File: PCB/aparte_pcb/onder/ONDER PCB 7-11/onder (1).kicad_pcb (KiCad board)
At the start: 2 copper layers, 170 x 170 mm, 77 parts, among them J1 Conn_01x04_Socket, J2 Conn_01x10_Socket, J3 Screw_Terminal_01x01, J4 Screw_Terminal_01x01, J5 Screw_Terminal_01x01, Q1 NPN, Q2 NPN, Q3 NPN

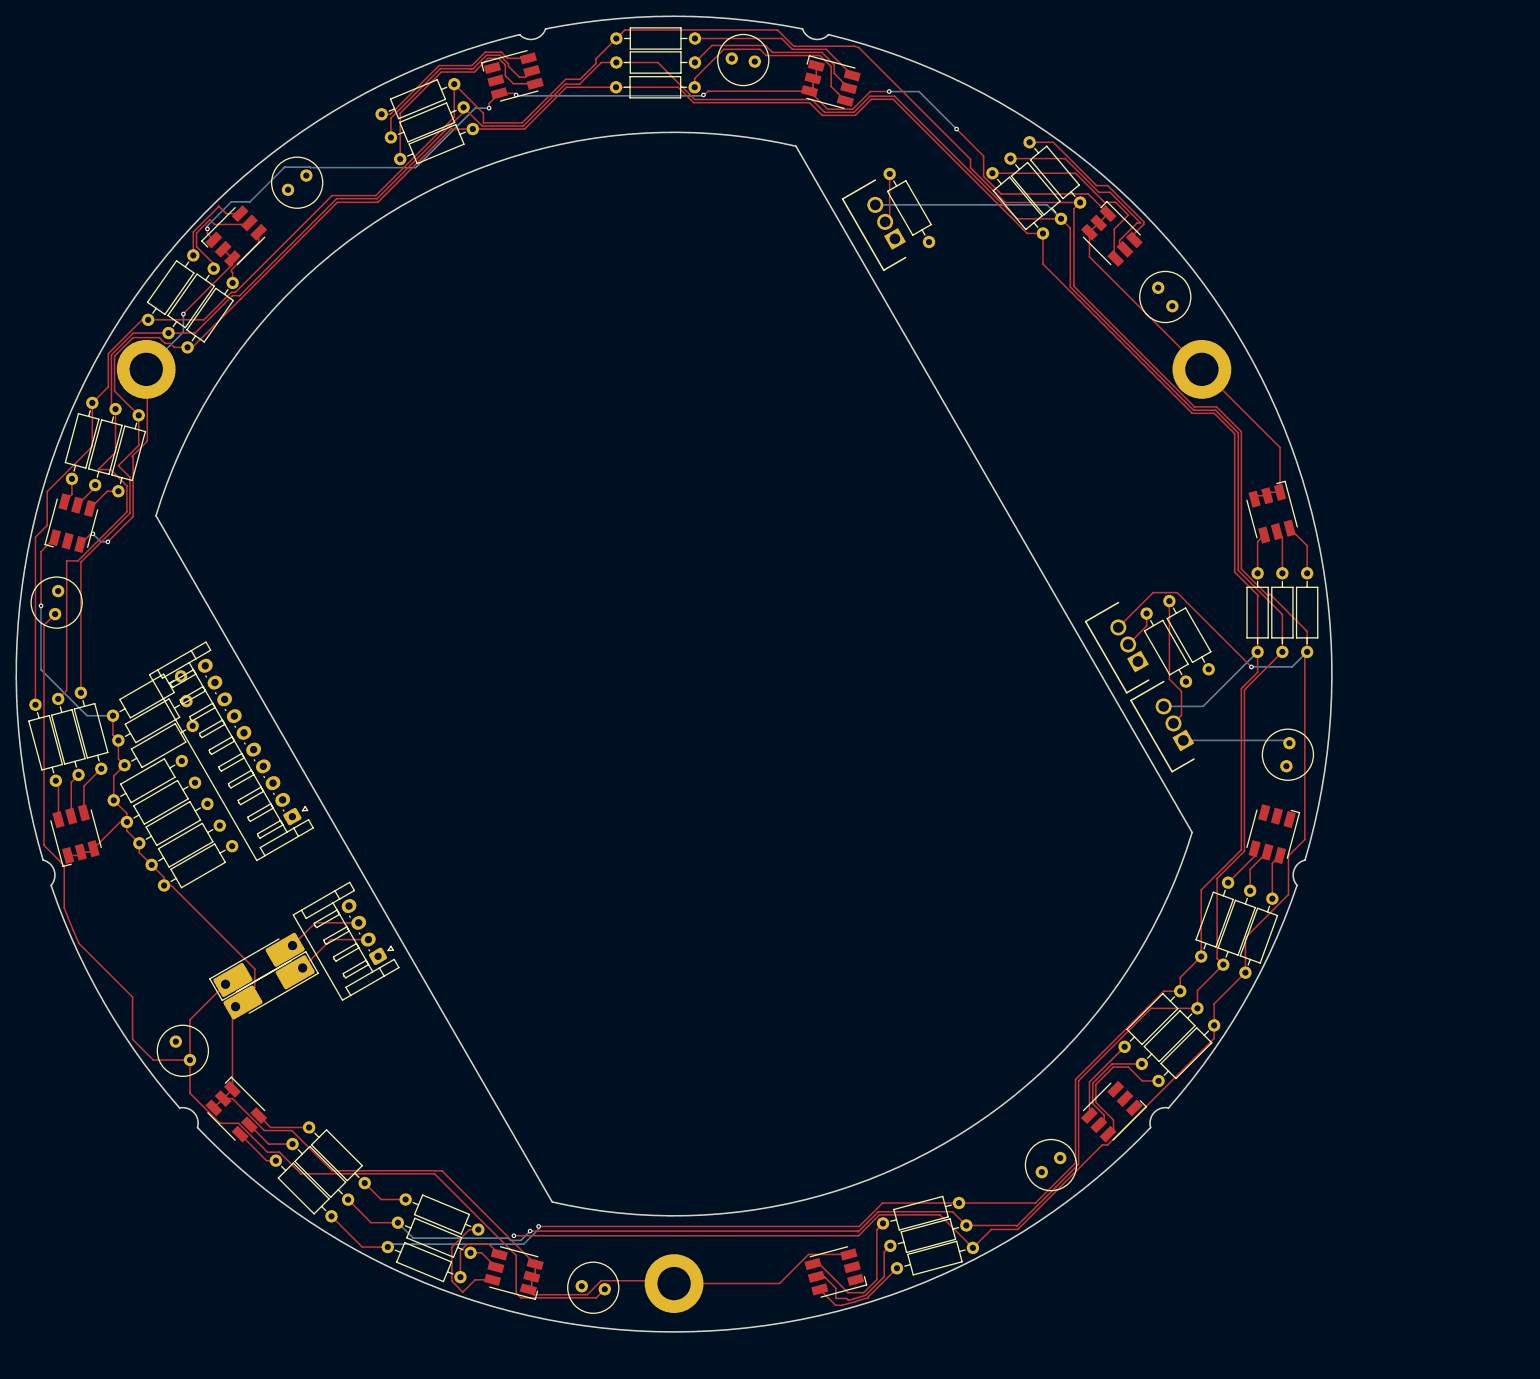
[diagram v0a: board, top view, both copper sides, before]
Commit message: af ready to check
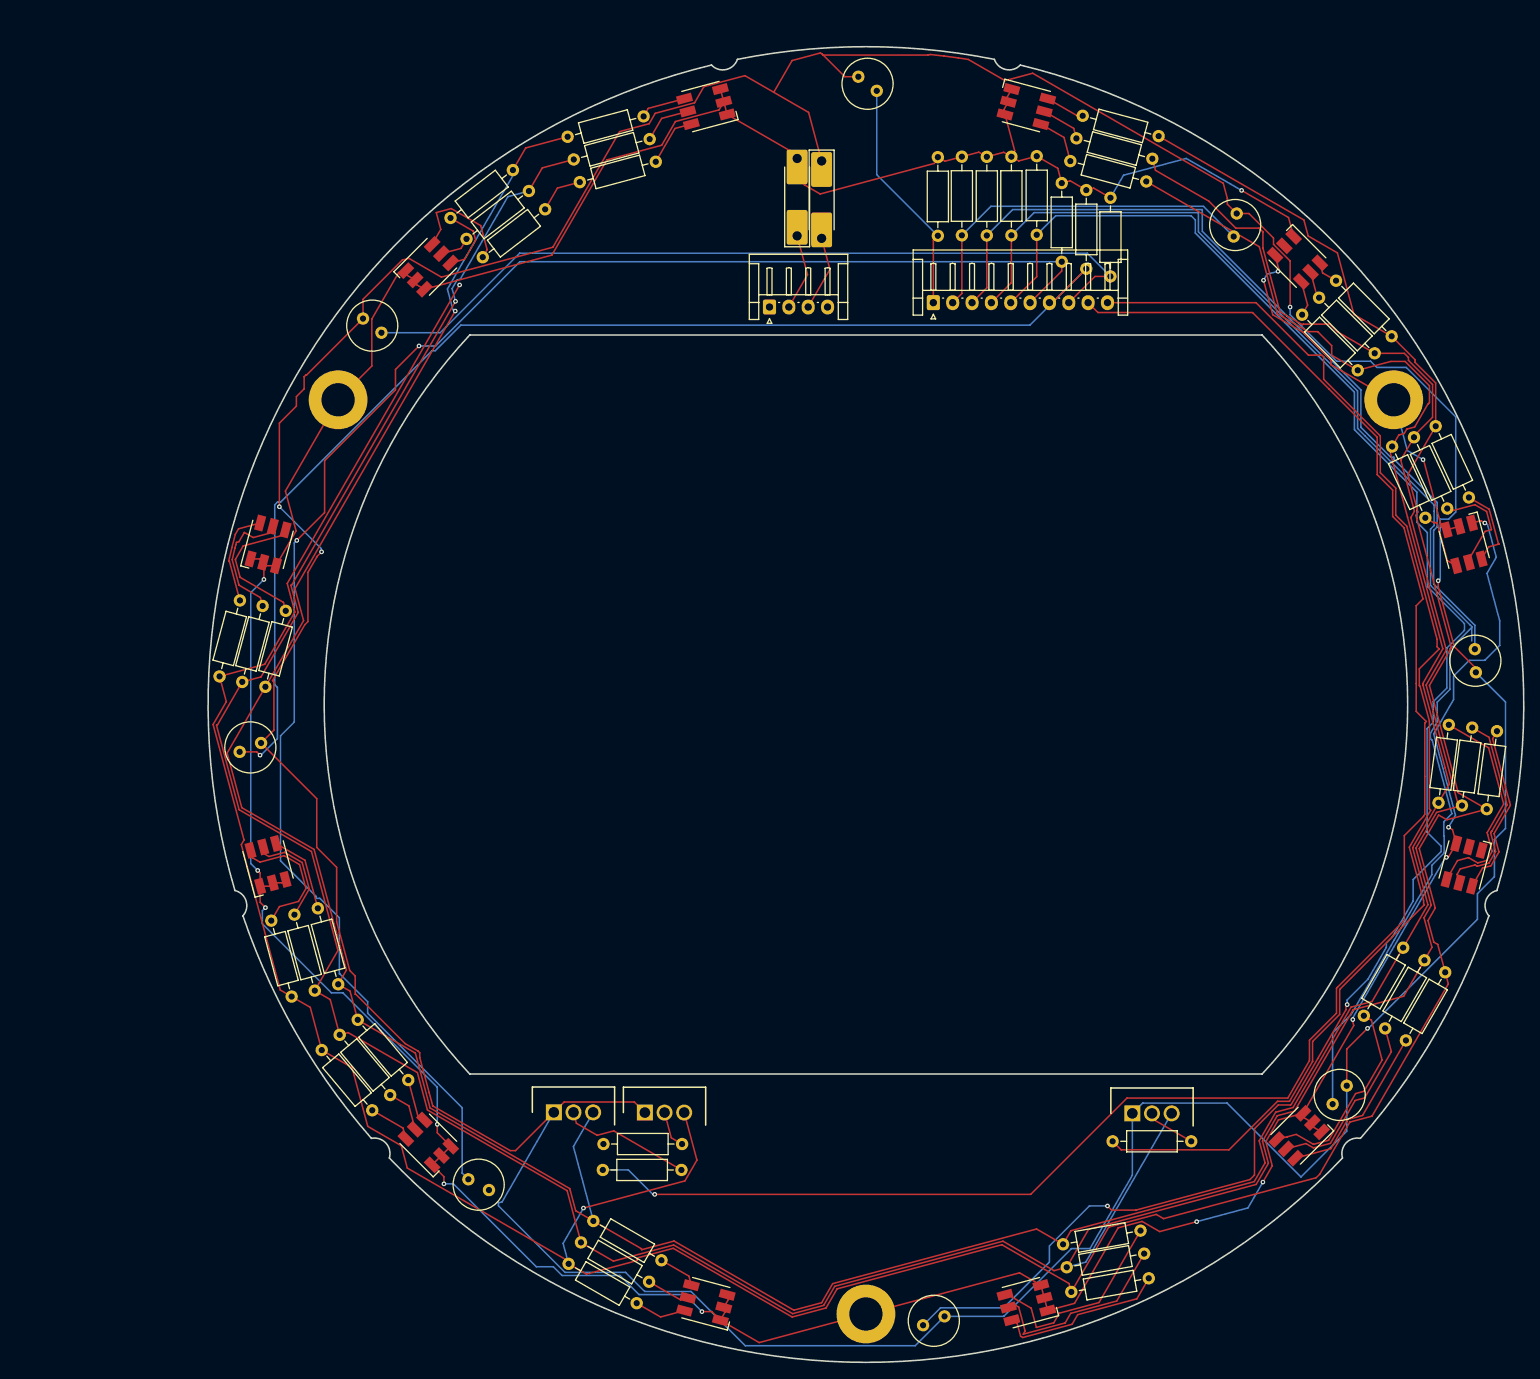
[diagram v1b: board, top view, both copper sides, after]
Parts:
- moved 220Ω_36 167.8 mm to (218.8, 81.3), turned to 115 degrees
- moved 220Ω_33 165.3 mm to (201.6, 53.3), turned to -45 degrees
- moved 220Ω_3 164.7 mm to (222.4, 111.5), turned to -97.5 degrees
- moved D12 163.6 mm to (218.2, 87.4), turned to -75 degrees
- moved 220Ω_35 162.4 mm to (216.0, 82.7), turned to 115 degrees
- moved D11 161.9 mm to (196.6, 50.5), turned to -45 degrees
- moved J5 161.2 mm to (209.1, 68.7), turned to -120 degrees
- moved 220Ω_32 160.0 mm to (199.4, 55.5), turned to -45 degrees
- moved D1 159.6 mm to (218.2, 128.8), turned to -105 degrees
- moved 220Ω_2 159.2 mm to (219.2, 111.0), turned to -97.5 degrees
- moved 220Ω_6 158.7 mm to (210.7, 151.5), turned to 60 degrees
- moved 220Ω_30 158.1 mm to (168.9, 32.0), turned to -15 degrees
- moved 220Ω_34 157.1 mm to (213.2, 83.9), turned to 115 degrees
- moved D10 154.6 mm to (161.6, 30.8), turned to -15 degrees
- moved 220Ω_31 154.6 mm to (197.2, 57.7), turned to -45 degrees
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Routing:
- net 5V: track 166.1 -> 615.7 mm, vias 0 -> 5
- net ROOD: track 0.00 -> 234.6 mm, vias 0 -> 1
- net pr5: track 0.00 -> 233.0 mm, vias 0 -> 2
- net pr6: track 0.00 -> 220.0 mm, vias 0 -> 2
- net pr4: track 0.00 -> 174.5 mm
- net GROEN: track 0.00 -> 167.2 mm
- net pr7: track 0.00 -> 160.4 mm, vias 0 -> 1
- net GND: track 438.7 -> 585.9 mm, vias 10 -> 16
- net pr3: track 0.00 -> 110.7 mm
- net pr8: track 0.00 -> 106.5 mm
- net pr2: track 0.00 -> 47.5 mm
- net pr1: track 0.00 -> 30.9 mm
- net Net-(Q2-E): track 481.2 -> 480.6 mm
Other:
- outline, holes or cut-outs redrawn
